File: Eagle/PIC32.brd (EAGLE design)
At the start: 50 x 50 mm, 22 parts

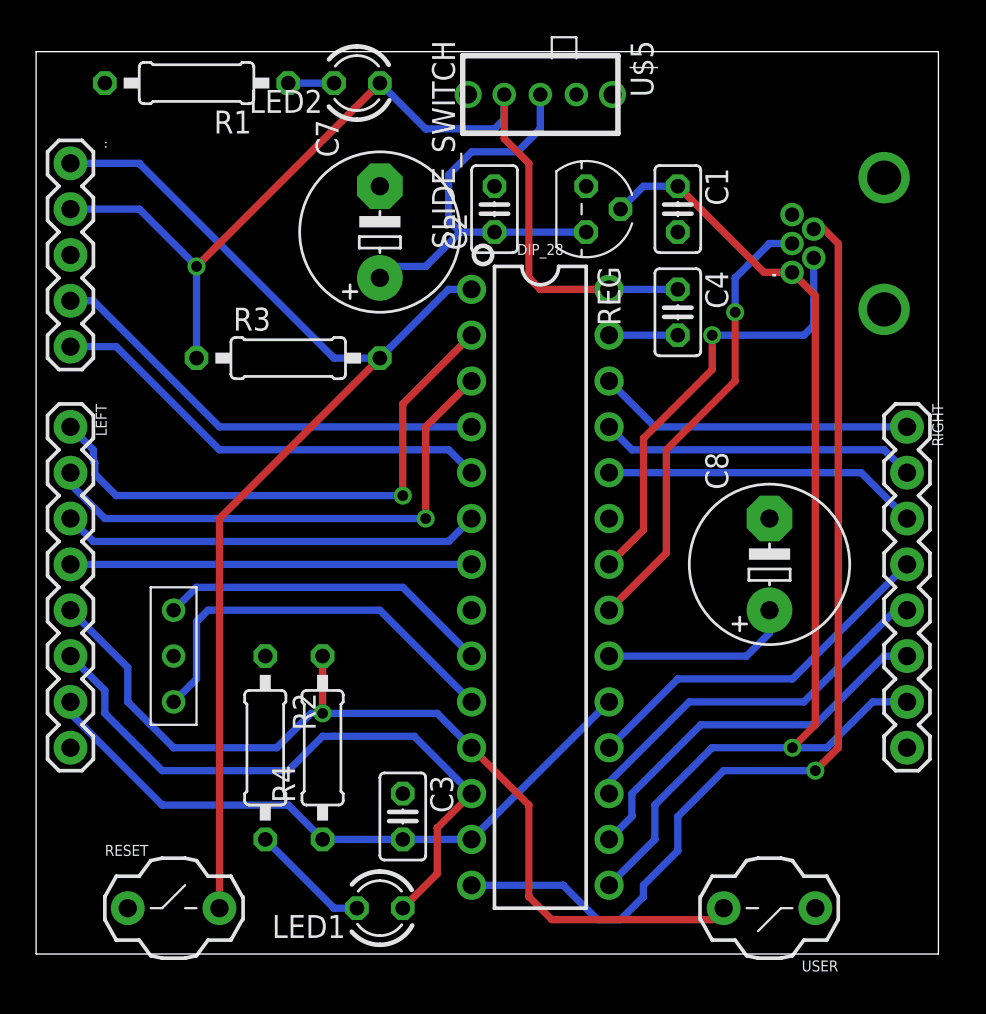
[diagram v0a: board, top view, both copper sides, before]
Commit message: uploading changes to eagle files and uploading HW3 with the Gerber files
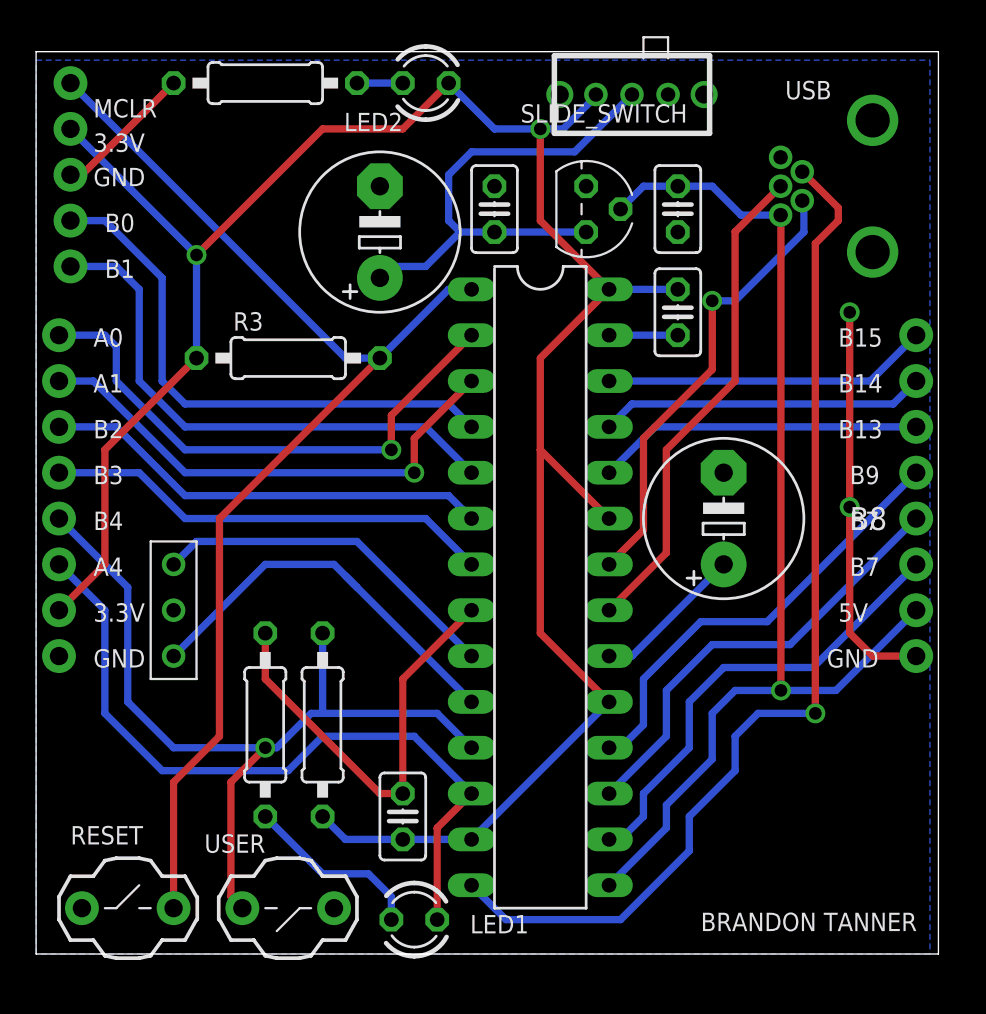
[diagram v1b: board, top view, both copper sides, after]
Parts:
- removed .: USB_MINI_B, meche-433:USB-MB-H
- added USB: USB_MINI_B, meche-433:USB-MB-H
- DIP_28: device meche-433:DIP28 -> meche-433:DIL28-3
- moved USER 26.7 mm to (16.5, 2.54)
- moved LEFT 5.12 mm to (1.27, 34.3)
- moved RIGHT 5.11 mm to (48.8, 34.3)
- moved U$5 5.08 mm to (33.0, 47.6)
- moved .. 4.45 mm to (1.91, 48.3)
- moved LED2 3.81 mm to (21.6, 48.3)
- moved R1 3.81 mm to (12.7, 48.3)
- moved C8 3.59 mm to (38.1, 24.1)
- moved RESET 2.54 mm to (2.54, 2.54)
- moved ... 2.54 mm to (7.62, 19.1)
- moved LED1 2.01 mm to (21.0, 1.91)
- moved R2 1.27 mm to (12.7, 12.7)
- moved R4 1.27 mm to (15.9, 12.7)
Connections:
- net D+: now also USB.D+; no longer ..D+
- net D-: now also USB.D-; no longer ..D-
- net GND: now also USB.GND; no longer ..GND
- net ID: now also USB.ID; no longer ..ID
- net VBUS: now also USB.VBUS; no longer ..VBUS
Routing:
- net GND: track 3.81 -> 58.1 mm, vias 0 -> 2
- net V3.3: track 93.1 -> 125.9 mm, vias 1 -> 2
- net A4: track 35.6 -> 40.8 mm
- net B0: track 25.1 -> 30.3 mm
- net B1: track 25.1 -> 29.9 mm
- net B4: track 52.4 -> 47.8 mm
- net B9: track 20.7 -> 24.8 mm
- net B7: track 21.5 -> 25.6 mm
- net N$4: track 24.0 -> 27.9 mm
- net B8: track 21.1 -> 24.8 mm
- net N$14: track 6.66 -> 10.1 mm
- net MCLR: track 62.4 -> 65.3 mm
- net B3: track 22.2 -> 25.0 mm
- net VCAP: track 10.7 -> 8.45 mm
- net D+: track 25.3 -> 27.4 mm, vias 1 -> 0
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- added copper zone on layer 16, net GND
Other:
- board text added: "3.3V"
- board text added: "5V"
- board text added: "A0"
- board text added: "A1"
- board text added: "A4"
- board text added: "B0"
- board text added: "B1"
- board text added: "B13"
- board text added: "B14"
- board text added: "B15"
- board text added: "B2"
- board text added: "B3"
- board text added: "B4"
- board text added: "B7"
- board text added: "B8"
- board text added: "B9"
- board text added: "BRANDON TANNER"
- board text added: "GND"
- board text added: "MCLR"
